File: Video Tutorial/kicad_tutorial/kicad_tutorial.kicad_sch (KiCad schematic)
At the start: 46 parts, among them J1 Screw_Terminal_01x02, J2 SWD, J3 Conn_01x04, J4 Conn_01x04, J5 USB_B_Micro, Q1 AO3401A, SW1 SW_SPDT, U1 STM32F405RGT6, U2 USBLC6-2SC6, Y1 16MHz

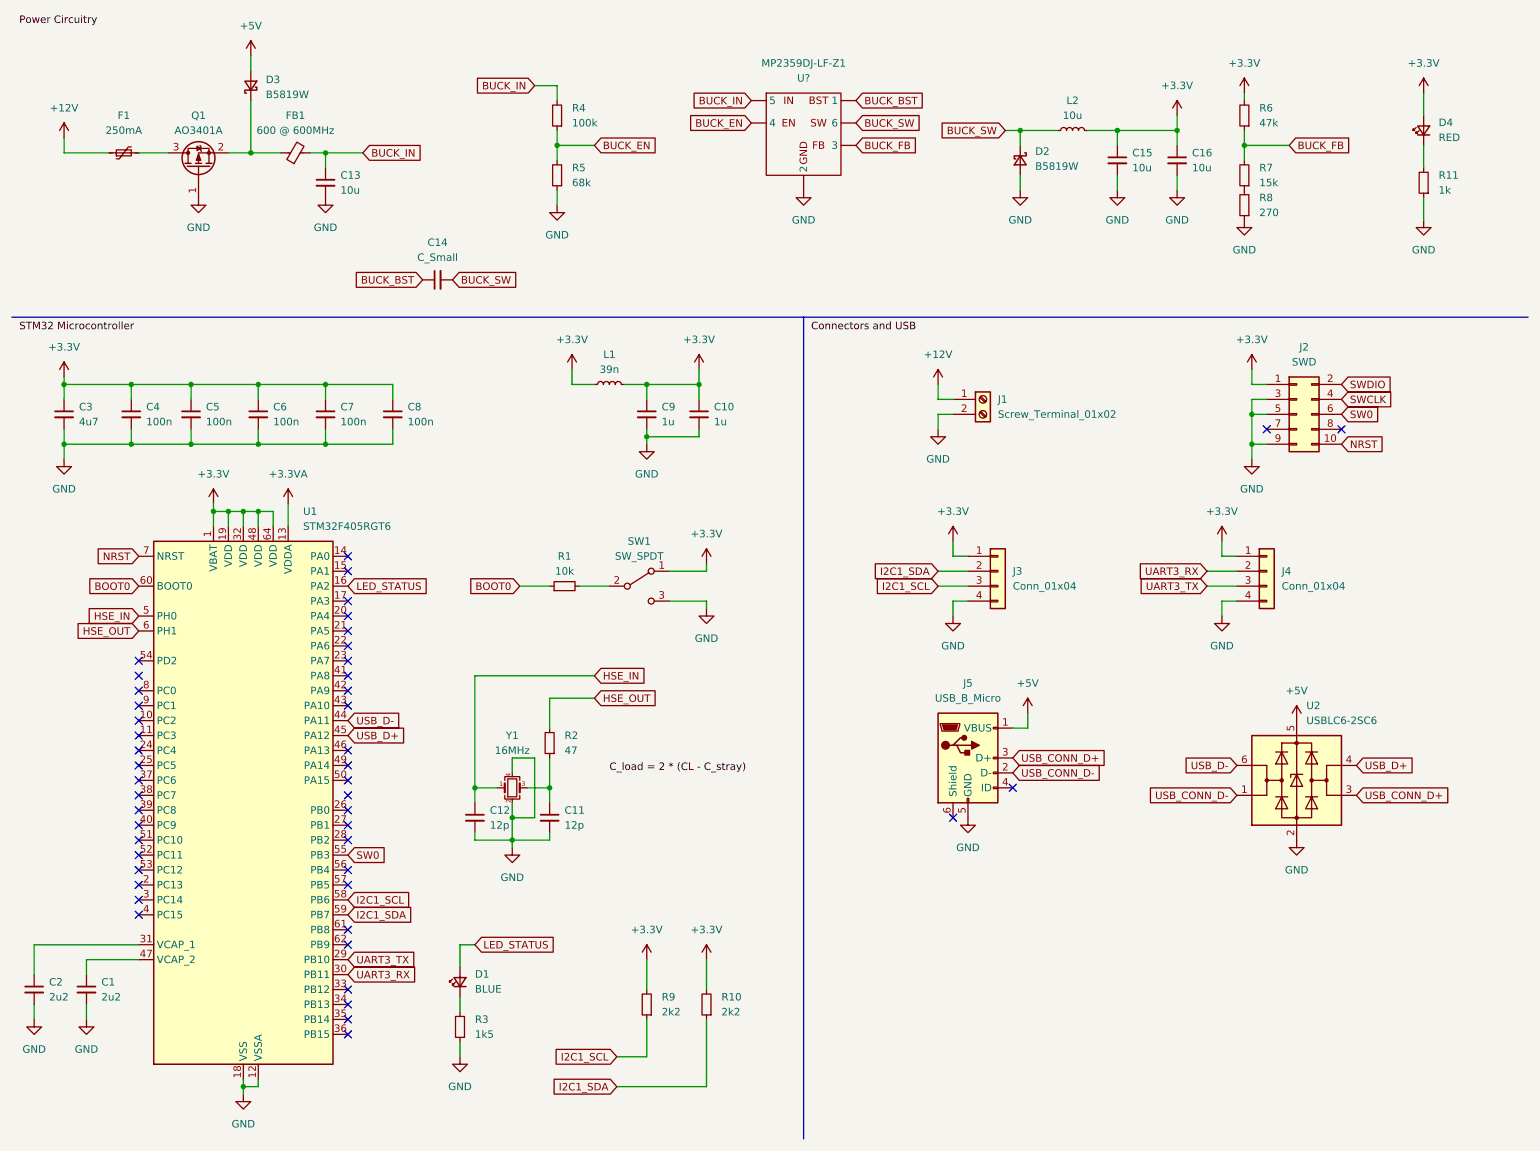
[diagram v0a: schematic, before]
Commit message: Added notes for Chapter: Design Rules
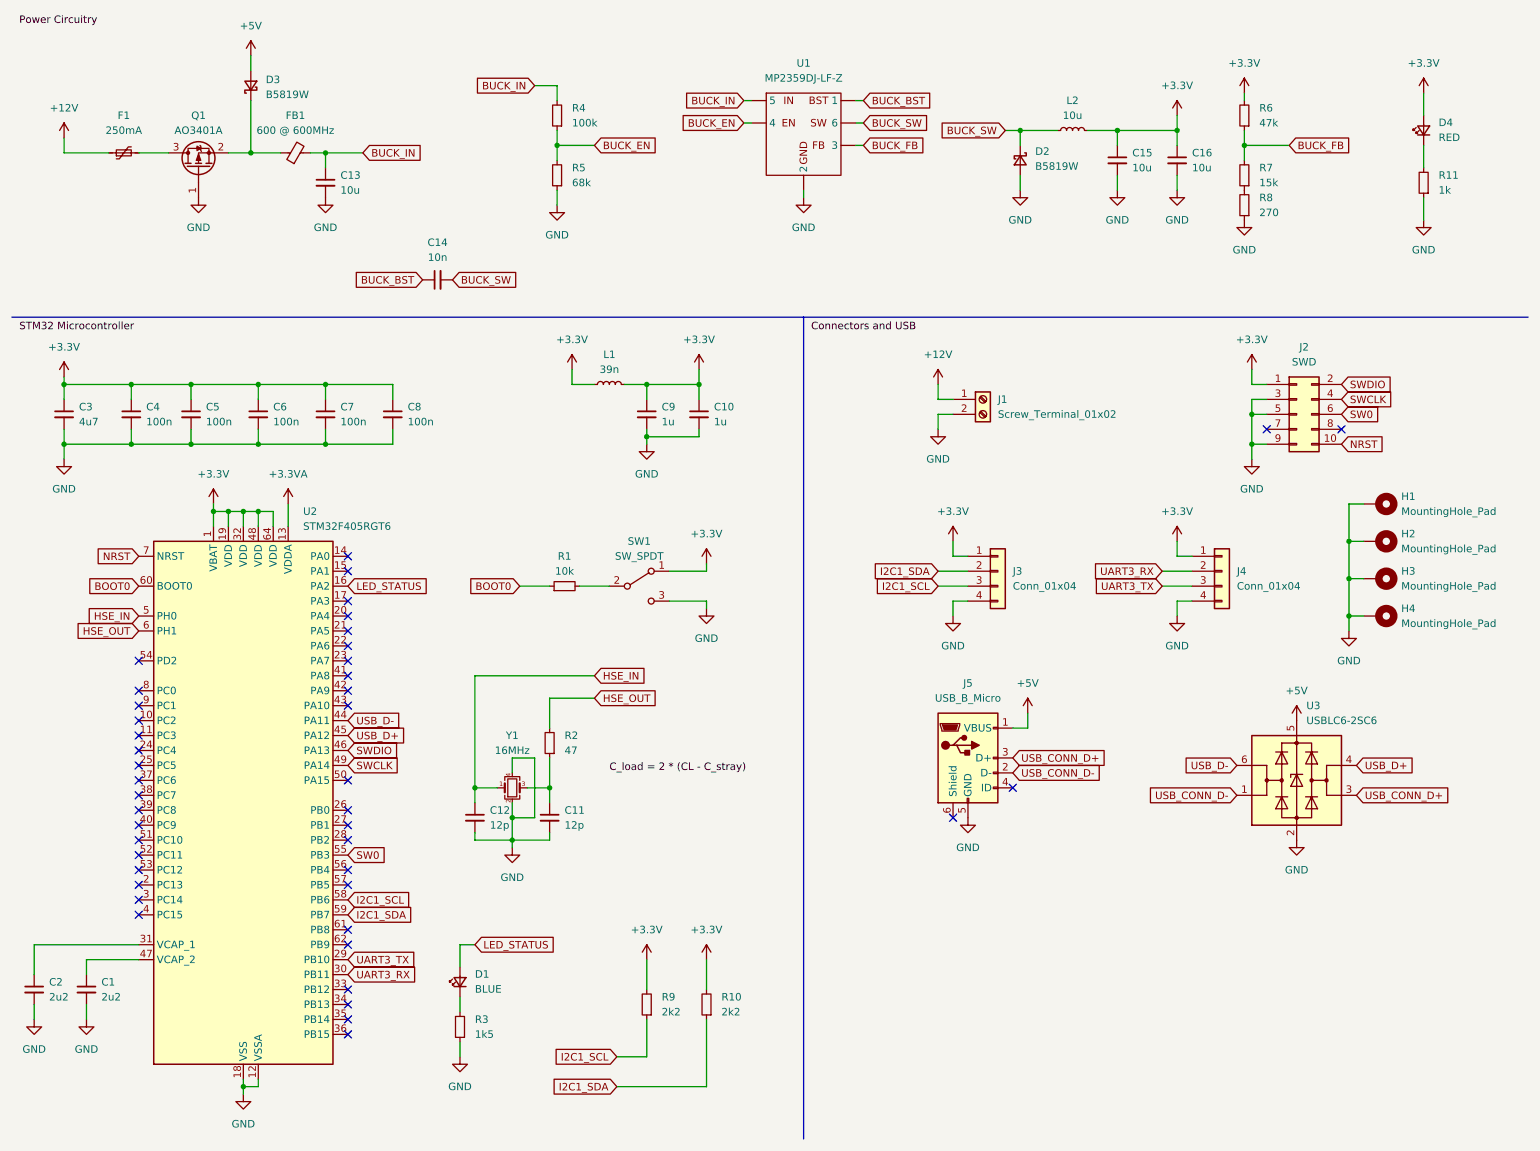
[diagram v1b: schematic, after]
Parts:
- added H1, H2, H3, H4: MountingHole_Pad, MountingHole:MountingHole_4.3mm_M4_Pad_Via, symbol Mechanical:MountingHole_Pad
- C1, C2, C3: footprint (none) -> Capacitor_SMD:C_0603_1608Metric
- C10, C11, C12, C4, C5, C6, C7, C8, C9: footprint (none) -> Capacitor_SMD:C_0402_1005Metric
- C13, C15, C16: footprint (none) -> Capacitor_SMD:C_1206_3216Metric
- C14: value C_Small -> 10n; footprint (none) -> Capacitor_SMD:C_0603_1608Metric
- D1, D4: footprint (none) -> LED_SMD:LED_0603_1608Metric
- D2, D3: footprint (none) -> Diode_SMD:D_SOD-123
- F1: footprint (none) -> Fuse:Fuse_1206_3216Metric
- FB1: footprint (none) -> Inductor_SMD:L_0805_2012Metric
- J1: footprint (none) -> TerminalBlock_Phoenix:TerminalBlock_Phoenix_PT-1,5-2-3.5-H_1x02_P3.50mm_Horizontal
- J2: footprint (none) -> Connector_PinHeader_1.27mm:PinHeader_2x05_P1.27mm_Vertical_SMD
- J3, J4: footprint (none) -> Connector_Molex:Molex_PicoBlade_53048-0410_1x04_P1.25mm_Horizontal
- J5: footprint (none) -> Connector_USB:USB_Micro-B_GCT_USB3076-30-A
- L1: footprint (none) -> Inductor_SMD:L_0402_1005Metric
- L2: footprint (none) -> Inductor_SMD:L_Sunlord_MWSA0518S
- R1, R10, R2, R9: footprint (none) -> Resistor_SMD:R_0402_1005Metric
- R11, R3, R4, R5, R6, R7, R8: footprint (none) -> Resistor_SMD:R_0603_1608Metric
- SW1: footprint (none) -> Button_Switch_SMD:SW_SPDT_PCM12
- U1: renamed from MP2359DJ-LF-Z1; value U? -> MP2359DJ-LF-Z; footprint (none) -> Package_TO_SOT_SMD:SOT-23-6
- Y1: footprint (none) -> Crystal:Crystal_SMD_3225-4Pin_3.2x2.5mm
- renumbered U1 to U2, U2 to U3
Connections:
- net GND: now also H1.1, H2.1, H3.1, H4.1
- net SWCLK: now also U2.49 (PA14)
- net SWDIO: now also U2.46 (PA13)
- no-connect marks 47 -> 43
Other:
- moved on the sheet: J4
